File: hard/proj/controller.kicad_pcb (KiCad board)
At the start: 2 copper layers, 35 x 70 mm, 49 parts, among them J1 microUSB, J2 EXT1, J3 EXT2, J4 EXT3, J5 EXT4, J6 UART, M1 MountingHole_3mm_Pad_Via, M2 MountingHole_3mm, M3 MountingHole_3mm_Pad_Via, M4 MountingHole_3mm_Pad_Via, Q1 BC848B, Q2 BC848B, Q3 BC848B, Q4 BC848B, SW1 RESET, SW2 FLASH, U1 LM3940, U2 ESP-07v2

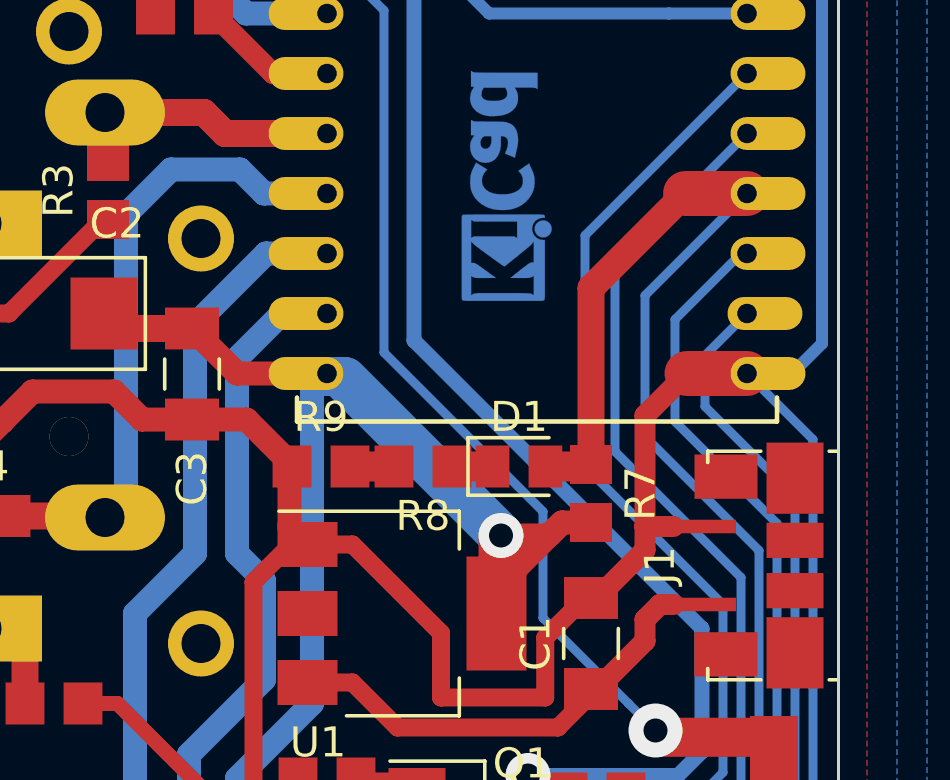
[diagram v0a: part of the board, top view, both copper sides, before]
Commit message: fixing errors
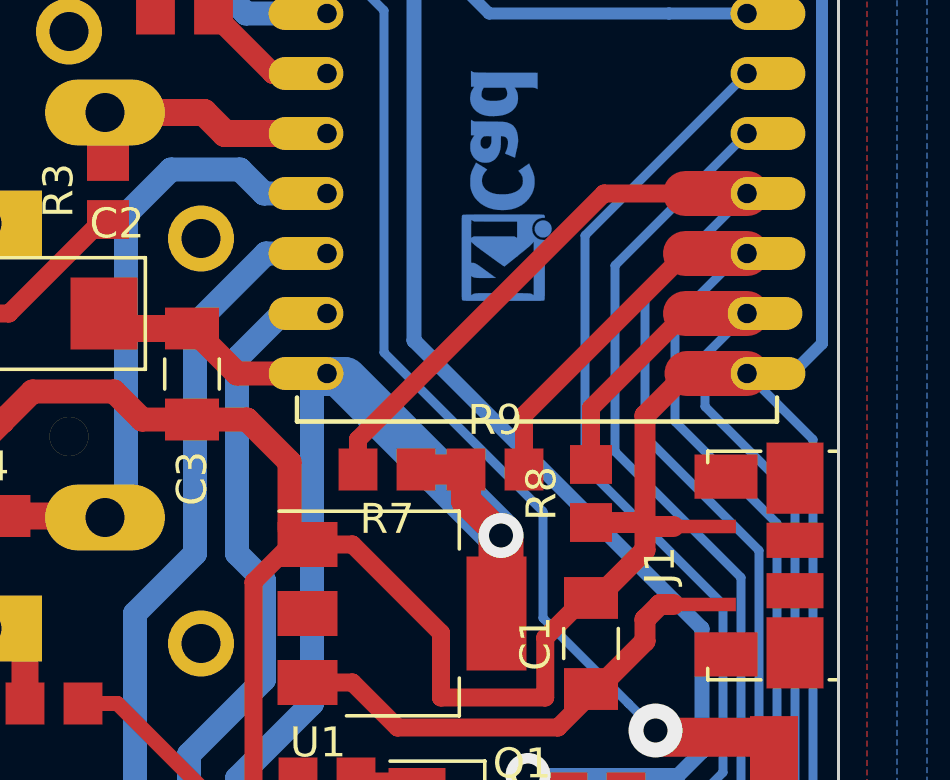
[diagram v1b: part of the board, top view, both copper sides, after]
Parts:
- removed D1: STATUS, LED_SMD:LED_0805_2012Metric_Pad1.12x1.40mm_HandSolder
- R8, R9: value 180 -> 10k
- moved R7 6.85 mm to (52.0, 120.2), turned to 180 degrees
- moved R9 5.80 mm to (55.6, 120.2)
- moved R8 5.67 mm to (58.8, 121.0), turned to 90 degrees
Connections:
- net /PC_RX renamed /UART_TX
- net /PC_TX renamed /UART_RX
- R7 pad 1: /FLASH -> +3V3
- R7 pad 2: +3V3 -> /FLASH
- R8 pad 1: Net-(D1-Pad1) -> GND
- R8 pad 2: Net-(R8-Pad2) -> /LED4_CTL
- R9 pad 1: GND -> +3V3
- R9 pad 2: Net-(R8-Pad2) -> /LED3_CTL
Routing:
- net /LED3_CTL: track 45.1 -> 56.6 mm
- net /LED4_CTL: track 47.4 -> 55.8 mm
- net /FLASH: track 85.6 -> 89.2 mm
- net GND: track 215.9 -> 218.0 mm
- net +3V3: track 217.7 -> 215.8 mm
- net Net-(R8-Pad2): track 1.47 -> 0.00 mm
- net Net-(D1-Pad1): track 1.35 -> 0.00 mm

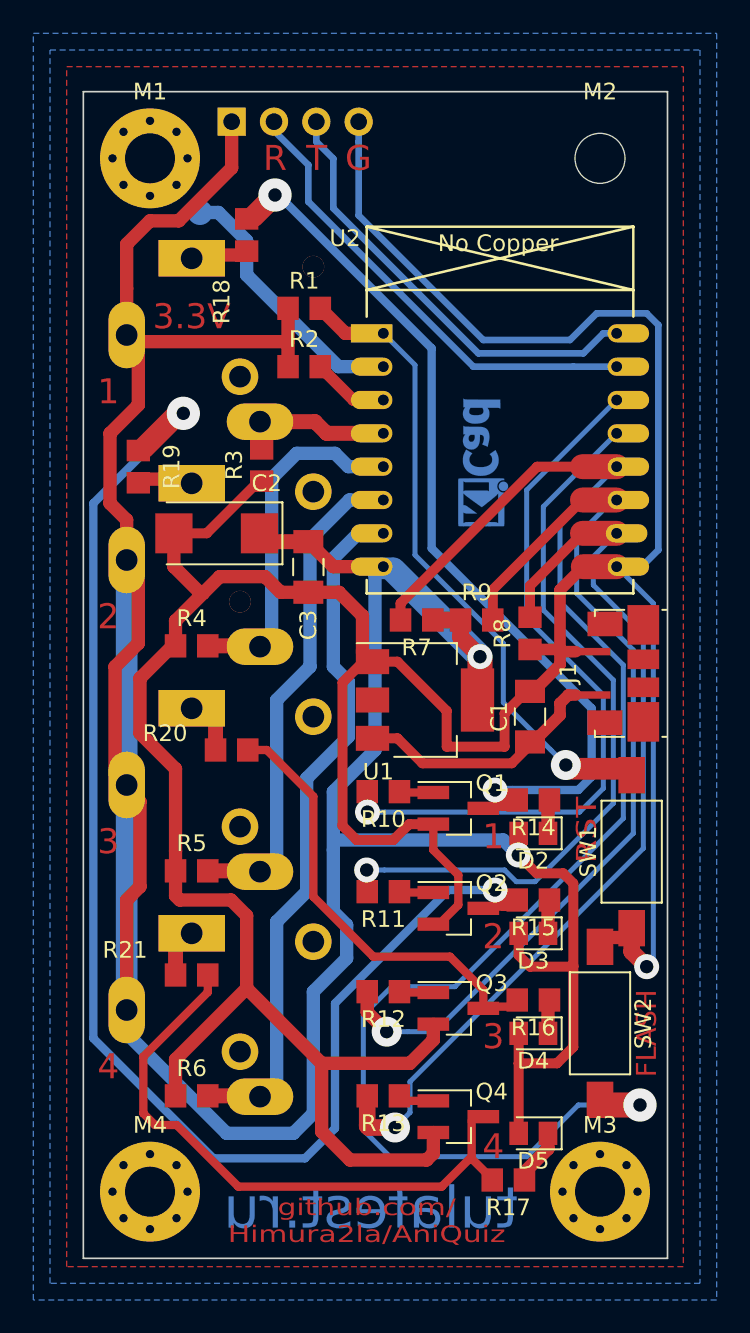
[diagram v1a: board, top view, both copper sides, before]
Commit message: fixing errors
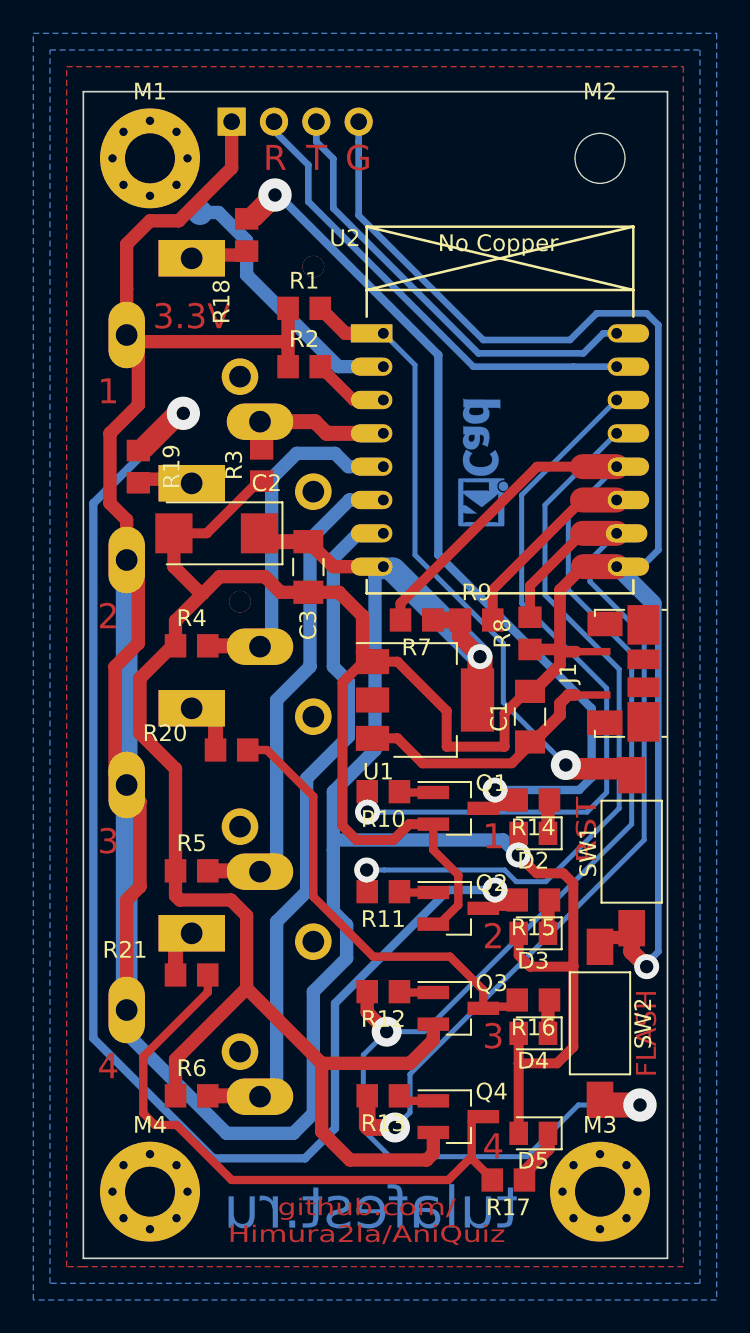
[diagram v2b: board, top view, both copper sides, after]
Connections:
- R7 pad 2: /FLASH -> /LED3_CTL
- R9 pad 2: /LED3_CTL -> /GPIO2_HIGH
- SW2 pad 2: /FLASH -> /LED3_CTL
- U2 pad 11: /LED3_CTL -> /GPIO2_HIGH
- U2 pad 12: /FLASH -> /LED3_CTL
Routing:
- net /FLASH: track 89.2 -> 0.00 mm, vias 1 -> 0
- net /LED3_CTL: track 56.6 -> 91.1 mm, vias 1 -> 2
- net /GPIO2_HIGH: track 0.00 -> 11.7 mm
- net /XLED2: track 3.03 -> 2.23 mm
- net /LED1_CTL: track 43.4 -> 44.1 mm
- net /LED2_CTL: track 44.1 -> 44.7 mm
